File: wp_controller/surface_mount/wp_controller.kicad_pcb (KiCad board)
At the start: 2 copper layers, 48.8 x 72.2 mm, 57 parts, among them J1 Pwr+, J10 SENSE, J2 Motor A, J3 Motor B, J4 UART_Device, J5 12v REG/R, J6 Conn_01x02, J7 Pwr-, J8 Conn_01x02, J9 Conn_01x02, Q1 Q_NMOS_GDS, Q2 Q_NMOS_GDS, Q3 Q_NMOS_GDS, Q4 Q_NMOS_GDS, Q5 Q_NMOS_GDS, U1 NCP5106B, U2 cpc5001, U3 NCP5106B

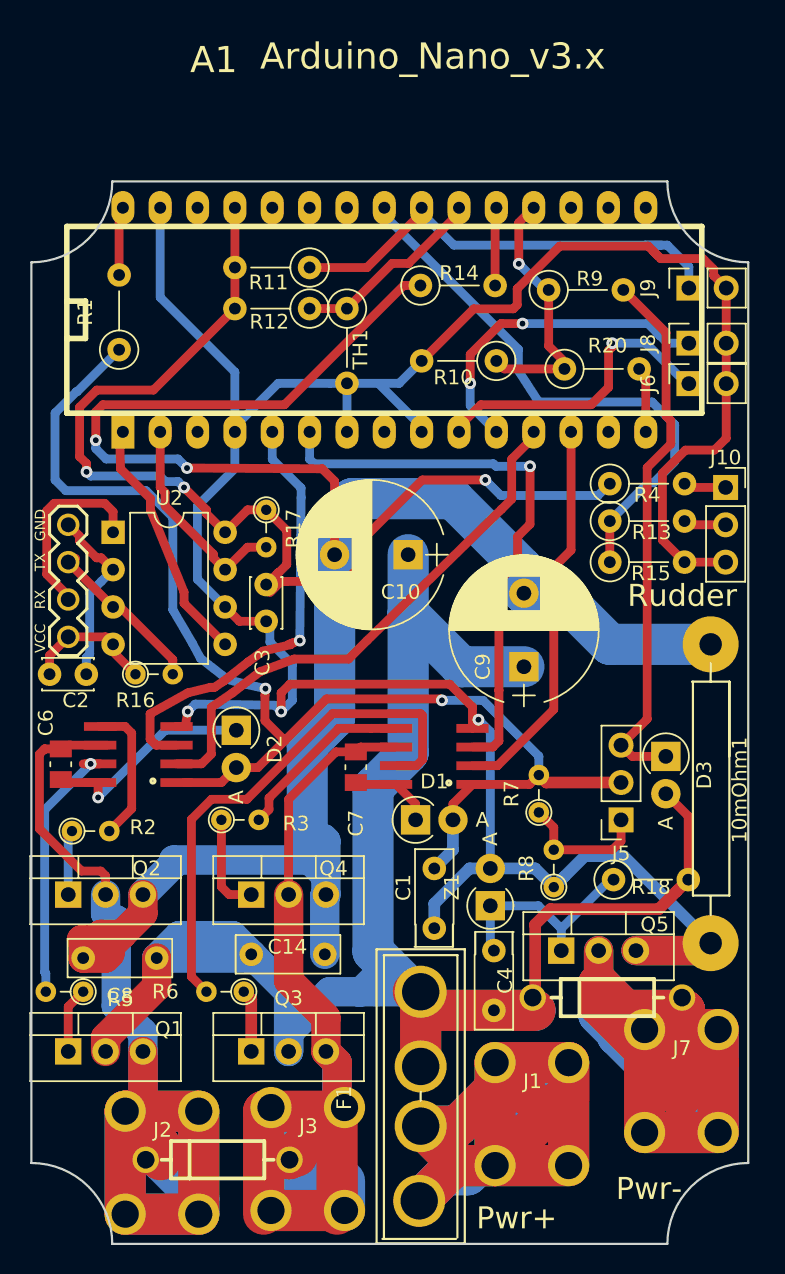
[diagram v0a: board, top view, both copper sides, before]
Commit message: update schematics
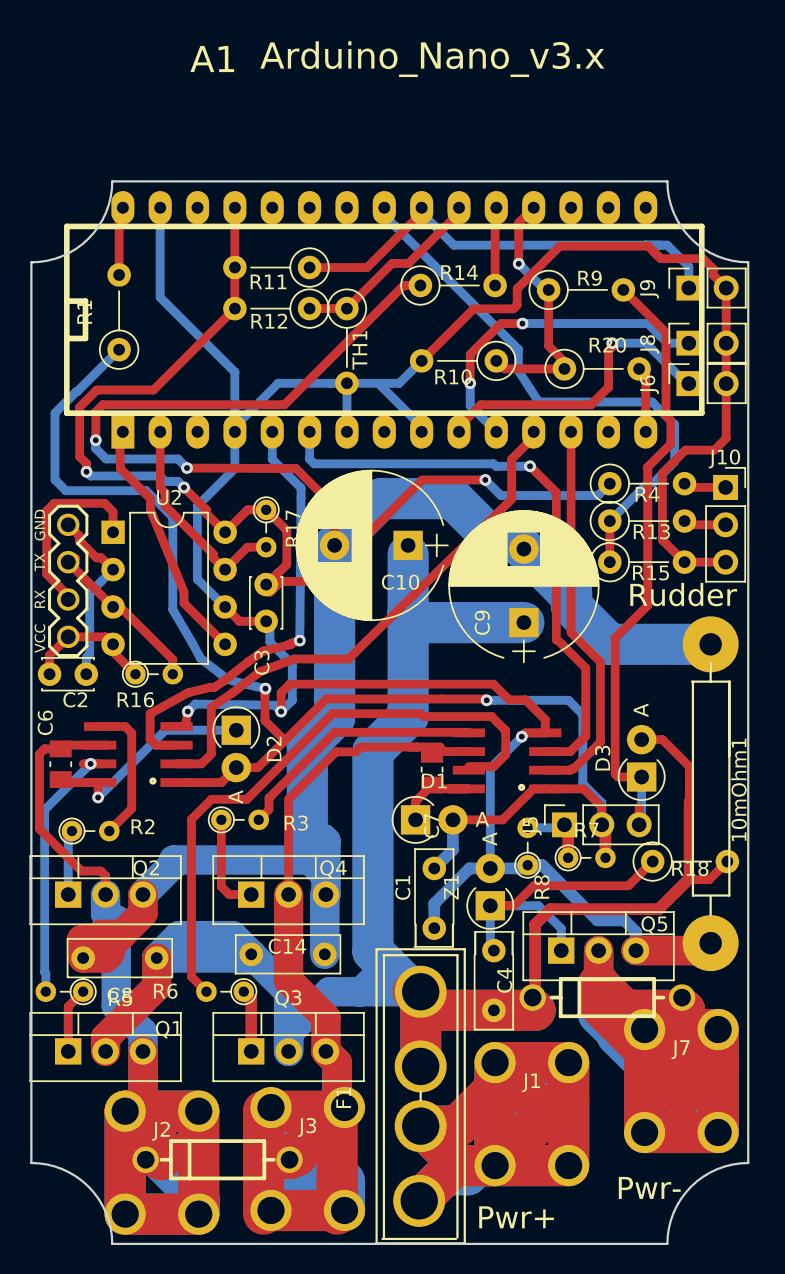
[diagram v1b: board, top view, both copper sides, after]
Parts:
- moved C7 5.19 mm to (93.6, 90.8)
- moved U3 4.96 mm to (98.7, 90.2)
- moved J5 3.86 mm to (102.6, 94.6), turned to 90 degrees
- moved R7 3.68 mm to (102.9, 96.8), turned to 0 degrees
- moved C9 3.00 mm to (99.9, 80.8)
- moved R18 2.93 mm to (108.6, 97.1)
- moved R8 2.32 mm to (100.1, 97.3)
- moved D3 2.16 mm to (107.9, 91.3), turned to 90 degrees
- moved C10 0.63 mm to (92.0, 75.6)
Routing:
- net +12V: track 85.7 -> 95.8 mm
- net Net-(C4-Pad2): track 15.1 -> 22.4 mm
- net VCC: track 139.5 -> 146.7 mm
- net Net-(C7-Pad2): track 92.0 -> 97.6 mm
- net Net-(R6-Pad2): track 35.8 -> 41.4 mm
- net /sense/Power: track 37.1 -> 42.3 mm
- net Net-(R3-Pad2): track 12.4 -> 17.2 mm
- net Net-(J5-Pad1): track 9.22 -> 4.94 mm
- net /sense/Shunt: track 140.5 -> 137.2 mm
- net /sense/PWMBL: track 38.9 -> 40.3 mm
- net Net-(C7-Pad1): track 5.75 -> 6.80 mm
